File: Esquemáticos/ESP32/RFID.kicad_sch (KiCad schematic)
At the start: 1 part

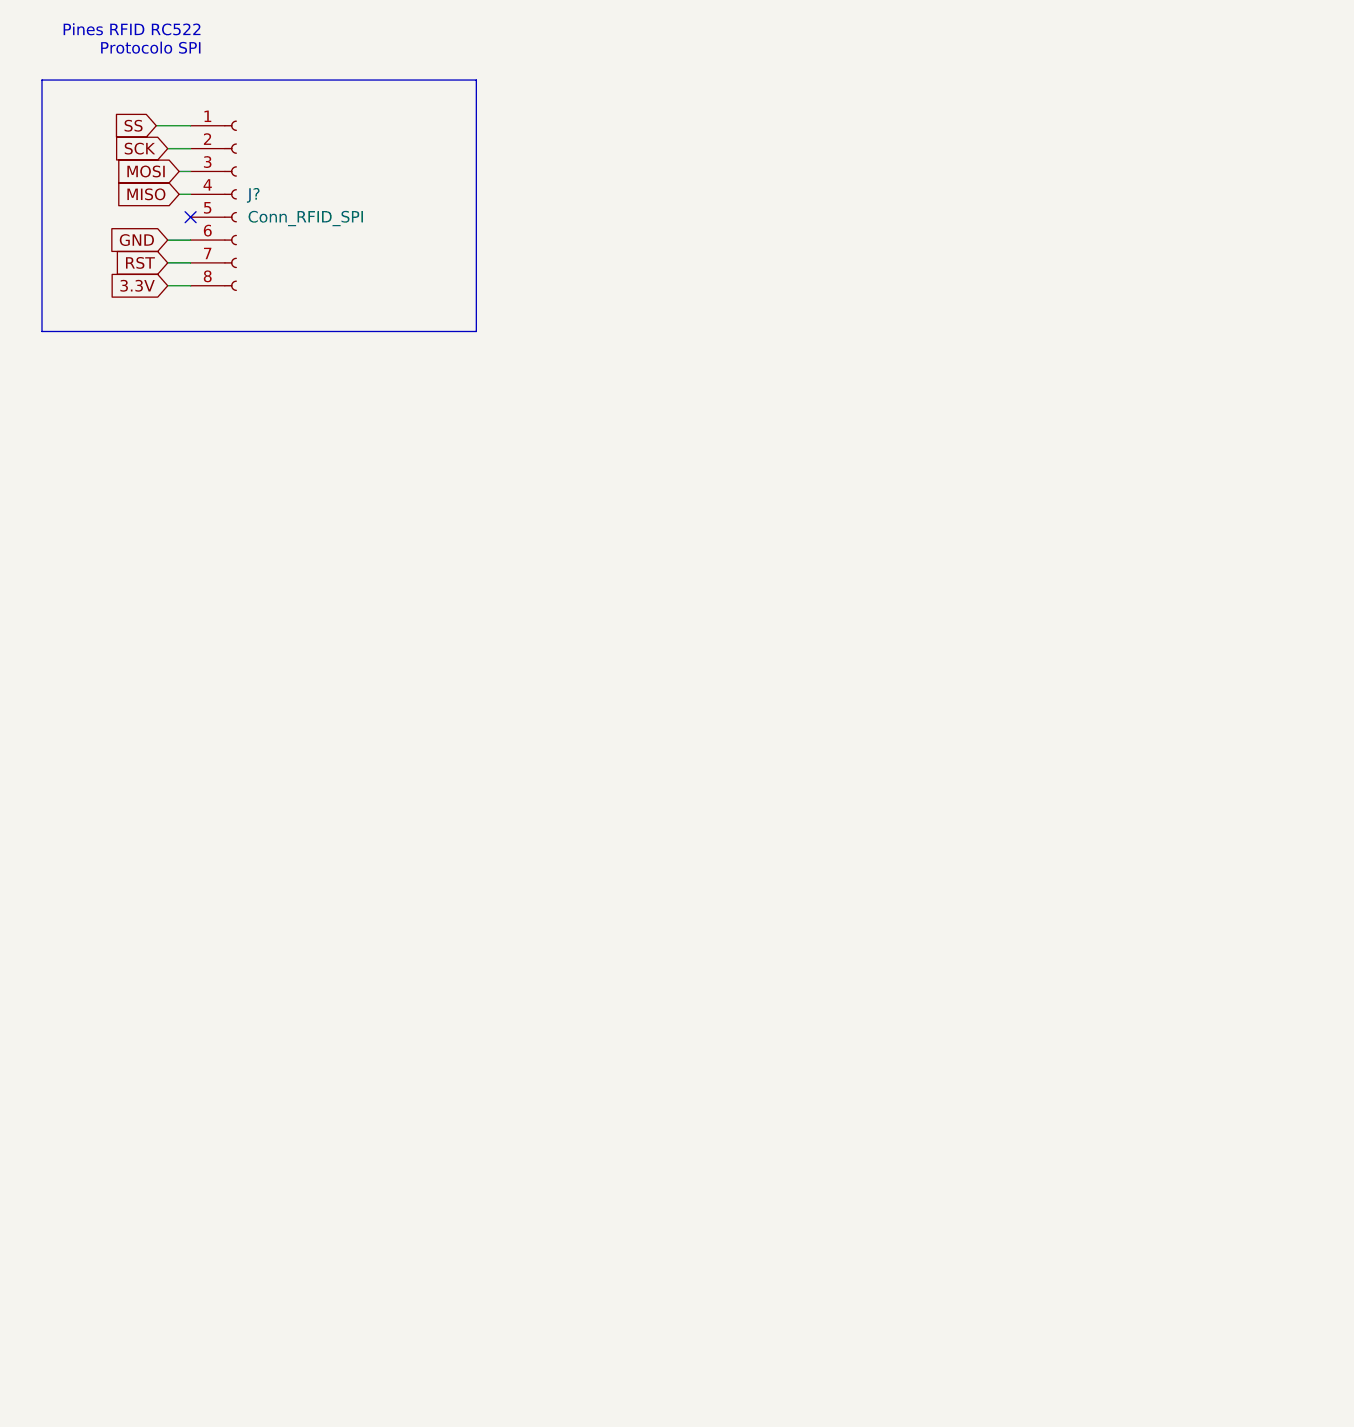
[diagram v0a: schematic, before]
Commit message: Cambios hechos al esquemático, faltan detalles
Revisar el discord para dejar todo al día con el feedback de hoy
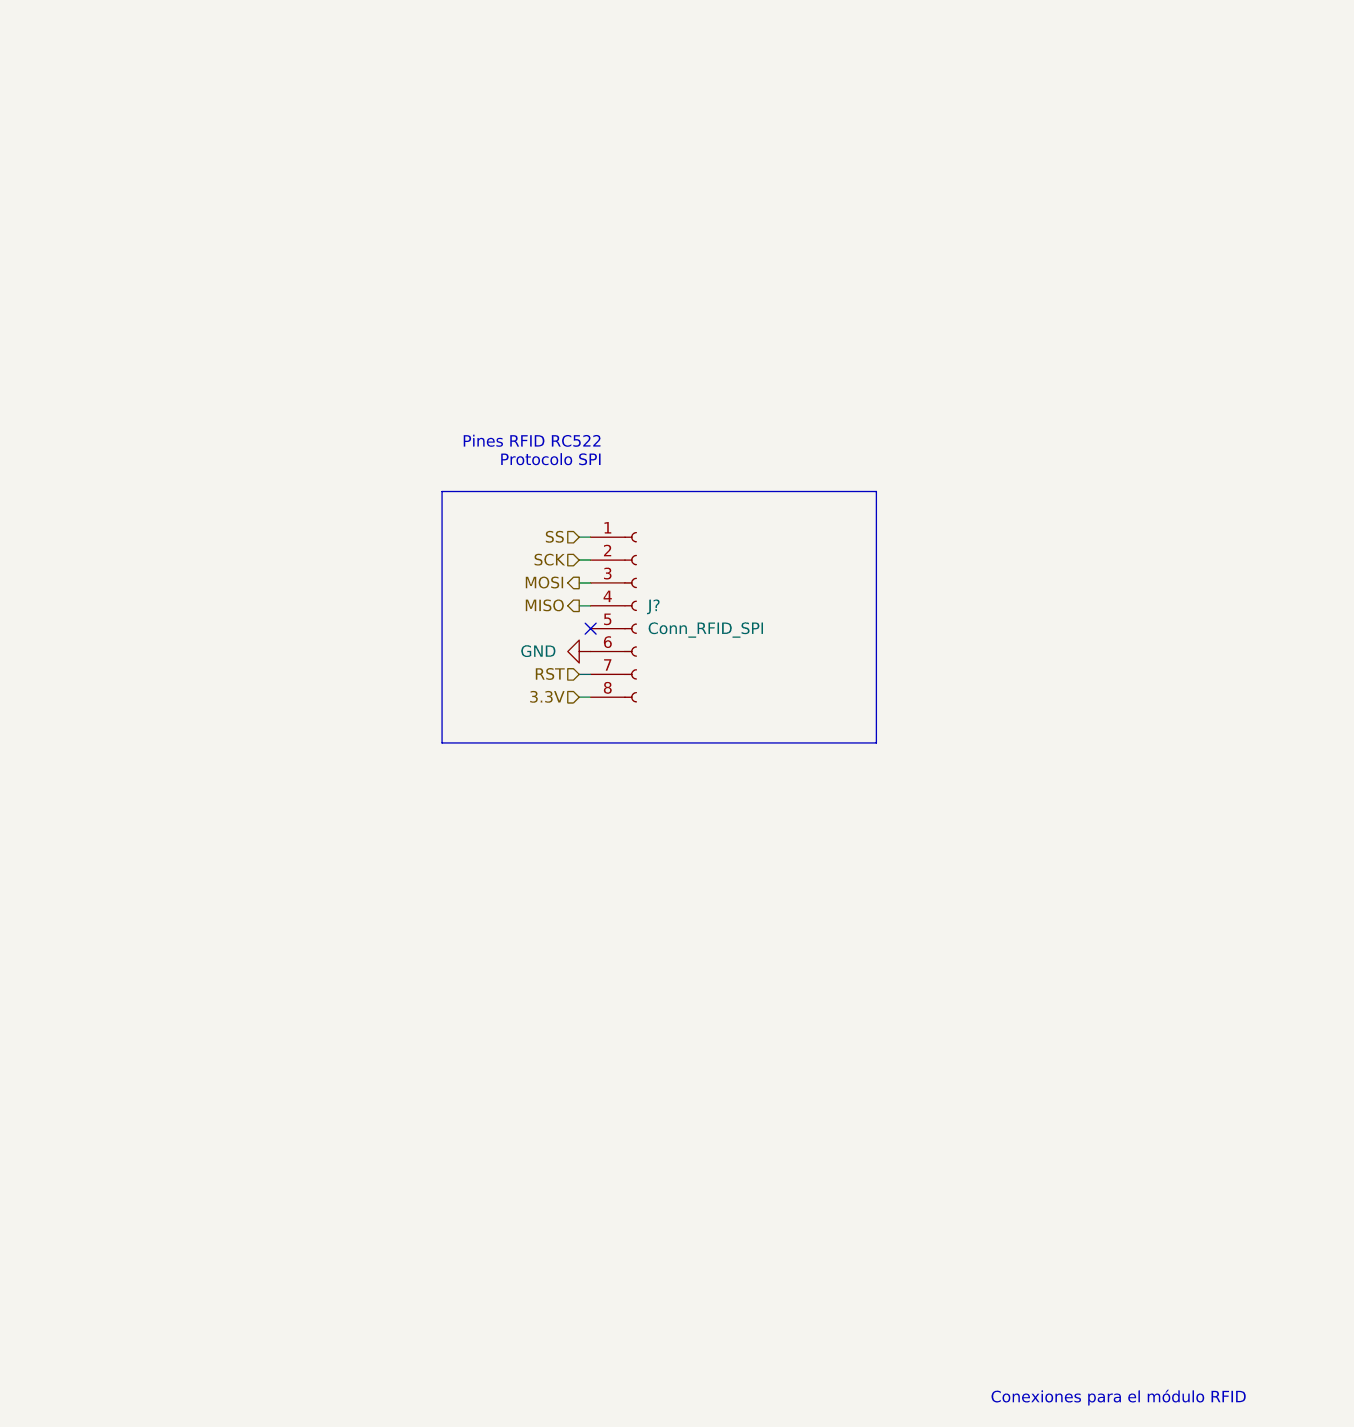
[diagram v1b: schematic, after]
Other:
- note added: "Conexiones para el módulo RFID"
- moved on the sheet: J?
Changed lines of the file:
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@@
 (kicad_sch (version 20211123) (generator eeschema)
   (paper "A4")
-  (no_connect (at 97.79 58.42))
-  (wire (pts (xy 95.25 50.8) (xy 97.79 50.8))
+  (no_connect (at 142.24 104.14))
+  (wire (pts (xy 140.97 96.52) (xy 142.24 96.52))
     (stroke (width 0) (type default) (color 0 0 0 0))
   )
-  (polyline (pts (xy 81.28 71.12) (xy 81.28 43.18))
+  (polyline (pts (xy 125.73 116.84) (xy 125.73 88.9))
     (stroke (width 0) (type default) (color 0 0 0 0))
   )
-  (wire (pts (xy 95.25 63.5) (xy 97.79 63.5))
+  (wire (pts (xy 140.97 109.22) (xy 142.24 109.22))
     (stroke (width 0) (type default) (color 0 0 0 0))
   )
-  (polyline (pts (xy 129.54 71.12) (xy 81.28 71.12))
+  (polyline (pts (xy 173.99 116.84) (xy 125.73 116.84))
     (stroke (width 0) (type default) (color 0 0 0 0))
   )
-  (wire (pts (xy 95.25 66.04) (xy 97.79 66.04))
+  (wire (pts (xy 140.97 111.76) (xy 142.24 111.76))
     (stroke (width 0) (type default) (color 0 0 0 0))
   )
-  (polyline (pts (xy 129.54 43.18) (xy 129.54 71.12))
+  (polyline (pts (xy 173.99 88.9) (xy 173.99 116.84))
     (stroke (width 0) (type default) (color 0 0 0 0))
   )
-  (wire (pts (xy 96.52 55.88) (xy 97.79 55.88))
+  (wire (pts (xy 140.97 101.6) (xy 142.24 101.6))
     (stroke (width 0) (type default) (color 0 0 0 0))
   )
-  (polyline (pts (xy 81.28 43.18) (xy 129.54 43.18))
+  (polyline (pts (xy 125.73 88.9) (xy 173.99 88.9))
     (stroke (width 0) (type default) (color 0 0 0 0))
   )
-  (wire (pts (xy 96.52 53.34) (xy 97.79 53.34))
+  (wire (pts (xy 140.97 99.06) (xy 142.24 99.06))
     (stroke (width 0) (type default) (color 0 0 0 0))
   )
-  (wire (pts (xy 95.25 60.96) (xy 97.79 60.96))
+  (wire (pts (xy 140.97 93.98) (xy 142.24 93.98))
     (stroke (width 0) (type default) (color 0 0 0 0))
   )
-  (wire (pts (xy 93.98 48.26) (xy 97.79 48.26))
-    (stroke (width 0) (type default) (color 0 0 0 0))
+  (text "Conexiones para el módulo RFID" (at 186.69 190.5 0)
+    (effects (font (size 1.27 1.27)) (justify left bottom))
   )
-  (text "Pines RFID RC522\nProtocolo SPI" (at 99.06 40.64 180)
+  (text "Pines RFID RC522\nProtocolo SPI" (at 143.51 86.36 180)
     (effects (font (size 1.27 1.27)) (justify right bottom))
   )
-  (global_label "MISO" (shape input) (at 96.52 55.88 180) (fields_autoplaced)
+  (hierarchical_label "MOSI" (shape output) (at 140.97 99.06 180)
     (effects (font (size 1.27 1.27)) (justify right))
-    (property "Referencias entre hojas" "${INTERSHEET_REFS}" (id 0) (at 89.5107 55.8006 0)
-      (effects (font (size 1.27 1.27)) (justify right) hide)
-    )
   )
-  (global_label "3.3V" (shape input) (at 95.25 66.04 180) (fields_autoplaced)
+  (hierarchical_label "MISO" (shape output) (at 140.97 101.6 180)
     (effects (font (size 1.27 1.27)) (justify right))
-    (property "Referencias entre hojas" "${INTERSHEET_REFS}" (id 0) (at 88.7245 65.9606 0)
-      (effects (font (size 1.27 1.27)) (justify right) hide)
-    )
   )
-  (global_label "SS" (shape input) (at 93.98 48.26 180) (fields_autoplaced)
+  (hierarchical_label "SS" (shape input) (at 140.97 93.98 180)
     (effects (font (size 1.27 1.27)) (justify right))
-    (property "Referencias entre hojas" "${INTERSHEET_REFS}" (id 0) (at 89.1479 48.1806 0)
-      (effects (font (size 1.27 1.27)) (justify right) hide)
-    )
   )
-  (global_label "MOSI" (shape input) (at 96.52 53.34 180) (fields_autoplaced)
+  (hierarchical_label "SCK" (shape input) (at 140.97 96.52 180)
     (effects (font (size 1.27 1.27)) (justify right))
-    (property "Referencias entre hojas" "${INTERSHEET_REFS}" (id 0) (at 89.5107 53.2606 0)
-      (effects (font (size 1.27 1.27)) (justify right) hide)
-    )
   )
-  (global_label "RST" (shape input) (at 95.25 63.5 180) (fields_autoplaced)
+  (hierarchical_label "3.3V" (shape input) (at 140.97 111.76 180)
     (effects (font (size 1.27 1.27)) (justify right))
-    (property "Referencias entre hojas" "${INTERSHEET_REFS}" (id 0) (at 89.3898 63.4206 0)
-      (effects (font (size 1.27 1.27)) (justify right) hide)
-    )
   )
-  (global_label "GND" (shape input) (at 95.25 60.96 180) (fields_autoplaced)
+  (hierarchical_label "RST" (shape input) (at 140.97 109.22 180)
     (effects (font (size 1.27 1.27)) (justify right))
-    (property "Referencias entre hojas" "${INTERSHEET_REFS}" (id 0) (at 88.9664 60.8806 0)
-      (effects (font (size 1.27 1.27)) (justify right) hide)
-    )
   )
-  (global_label "SCK" (shape input) (at 95.25 50.8 180) (fields_autoplaced)
-    (effects (font (size 1.27 1.27)) (justify right))
-    (property "Referencias entre hojas" "${INTERSHEET_REFS}" (id 0) (at 89.0874 50.7206 0)
-      (effects (font (size 1.27 1.27)) (justify right) hide)
-    )
-  )
-  (symbol (lib_id "Connector:Conn_01x08_Female") (at 102.87 55.88 0) (unit 1)
+  (symbol (lib_id "Connector:Conn_01x08_Female") (at 147.32 101.6 0) (unit 1)
     (in_bom yes) (on_board yes) (fields_autoplaced)
-    (property "Reference" "J?" (id 0) (at 104.14 55.8799 0)
+    (property "Reference" "J?" (id 0) (at 148.59 101.5999 0)
       (effects (font (size 1.27 1.27)) (justify left))
     )
-    (property "Value" "Conn_RFID_SPI" (id 1) (at 104.14 58.4199 0)
+    (property "Value" "Conn_RFID_SPI" (id 1) (at 148.59 104.1399 0)
       (effects (font (size 1.27 1.27)) (justify left))
     )
-    (property "Footprint" "" (id 2) (at 102.87 55.88 0)
+    (property "Footprint" "" (id 2) (at 147.32 101.6 0)
       (effects (font (size 1.27 1.27)) hide)
     )
-    (property "Datasheet" "~" (id 3) (at 102.87 55.88 0)
+    (property "Datasheet" "~" (id 3) (at 147.32 101.6 0)
       (effects (font (size 1.27 1.27)) hide)
     )
@@
     (pin "8")
   )
+  (symbol (lib_id "power:GND") (at 142.24 106.68 270) (unit 1)
+    (in_bom yes) (on_board yes) (fields_autoplaced)
+    (property "Reference" "#PWR?" (id 0) (at 135.89 106.68 0)
+      (effects (font (size 1.27 1.27)) hide)
+    )
+    (property "Value" "GND" (id 1) (at 138.43 106.6799 90)
+      (effects (font (size 1.27 1.27)) (justify right))
+    )
+    (property "Footprint" "" (id 2) (at 142.24 106.68 0)
+      (effects (font (size 1.27 1.27)) hide)
+    )
+    (property "Datasheet" "" (id 3) (at 142.24 106.68 0)
+      (effects (font (size 1.27 1.27)) hide)
+    )
+    (pin "1")
+  )
 )

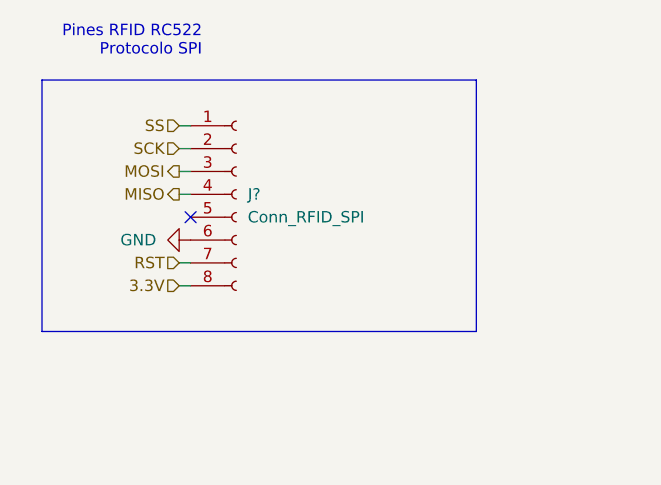
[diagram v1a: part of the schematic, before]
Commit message: actualización raul
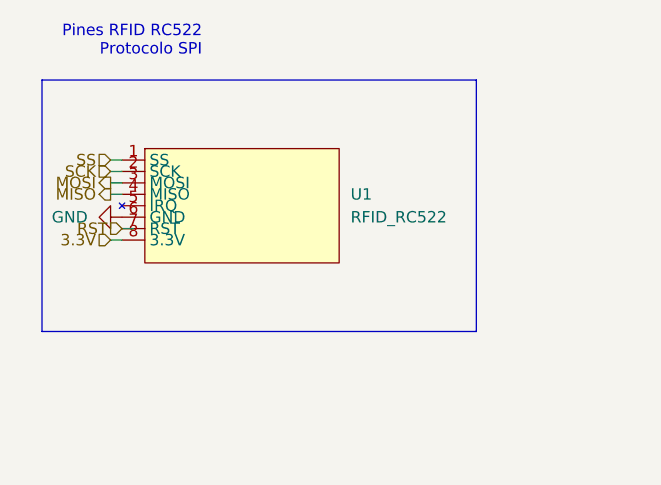
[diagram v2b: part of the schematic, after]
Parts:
- removed J?: Conn_RFID_SPI, symbol Connector:Conn_01x08_Female
- added U1: RFID_RC522, symbol libreria_raul:RFID_RC522
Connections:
- net 3.3V: now also U1.8 (3.3V)
- net GND: now also U1.6 (GND)
- net MISO: now also U1.4 (MISO)
- net MOSI: now also U1.3 (MOSI)
- net RST: now also U1.7 (RST)
- net SCK: now also U1.2 (SCK)
- net SS: now also U1.1 (SS)
- no-connect marks 1 -> 0
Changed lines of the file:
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@@
 (kicad_sch (version 20211123) (generator eeschema)
   (paper "A4")
-  (no_connect (at 142.24 104.14))
-  (wire (pts (xy 140.97 96.52) (xy 142.24 96.52))
+  (wire (pts (xy 133.35 99.06) (xy 134.62 99.06))
     (stroke (width 0) (type default) (color 0 0 0 0))
   )
@@
     (stroke (width 0) (type default) (color 0 0 0 0))
   )
-  (wire (pts (xy 140.97 109.22) (xy 142.24 109.22))
+  (wire (pts (xy 134.62 105.41) (xy 135.89 105.41))
     (stroke (width 0) (type default) (color 0 0 0 0))
   )
@@
     (stroke (width 0) (type default) (color 0 0 0 0))
   )
-  (wire (pts (xy 140.97 111.76) (xy 142.24 111.76))
+  (wire (pts (xy 133.35 106.68) (xy 134.62 106.68))
     (stroke (width 0) (type default) (color 0 0 0 0))
   )
@@
     (stroke (width 0) (type default) (color 0 0 0 0))
   )
-  (wire (pts (xy 140.97 101.6) (xy 142.24 101.6))
+  (wire (pts (xy 133.35 101.6) (xy 134.62 101.6))
     (stroke (width 0) (type default) (color 0 0 0 0))
   )
@@
     (stroke (width 0) (type default) (color 0 0 0 0))
   )
-  (wire (pts (xy 140.97 99.06) (xy 142.24 99.06))
+  (wire (pts (xy 133.35 100.33) (xy 134.62 100.33))
     (stroke (width 0) (type default) (color 0 0 0 0))
   )
-  (wire (pts (xy 140.97 93.98) (xy 142.24 93.98))
+  (wire (pts (xy 133.35 97.79) (xy 134.62 97.79))
     (stroke (width 0) (type default) (color 0 0 0 0))
   )
@@
     (effects (font (size 1.27 1.27)) (justify right bottom))
   )
-  (hierarchical_label "MOSI" (shape output) (at 140.97 99.06 180)
+  (hierarchical_label "MOSI" (shape output) (at 133.35 100.33 180)
     (effects (font (size 1.27 1.27)) (justify right))
   )
-  (hierarchical_label "MISO" (shape output) (at 140.97 101.6 180)
+  (hierarchical_label "MISO" (shape output) (at 133.35 101.6 180)
     (effects (font (size 1.27 1.27)) (justify right))
   )
-  (hierarchical_label "SS" (shape input) (at 140.97 93.98 180)
+  (hierarchical_label "SS" (shape input) (at 133.35 97.79 180)
     (effects (font (size 1.27 1.27)) (justify right))
   )
-  (hierarchical_label "SCK" (shape input) (at 140.97 96.52 180)
+  (hierarchical_label "SCK" (shape input) (at 133.35 99.06 180)
     (effects (font (size 1.27 1.27)) (justify right))
   )
-  (hierarchical_label "3.3V" (shape input) (at 140.97 111.76 180)
+  (hierarchical_label "3.3V" (shape input) (at 133.35 106.68 180)
     (effects (font (size 1.27 1.27)) (justify right))
   )
-  (hierarchical_label "RST" (shape input) (at 140.97 109.22 180)
+  (hierarchical_label "RST" (shape input) (at 134.62 105.41 180)
     (effects (font (size 1.27 1.27)) (justify right))
   )
-  (symbol (lib_id "Connector:Conn_01x08_Female") (at 147.32 101.6 0) (unit 1)
+  (symbol (lib_id "libreria_raul:RFID_RC522") (at 146.05 93.98 0) (unit 1)
     (in_bom yes) (on_board yes) (fields_autoplaced)
-    (property "Reference" "J?" (id 0) (at 148.59 101.5999 0)
+    (property "Reference" "U1" (id 0) (at 160.02 101.5999 0)
       (effects (font (size 1.27 1.27)) (justify left))
     )
-    (property "Value" "Conn_RFID_SPI" (id 1) (at 148.59 104.1399 0)
+    (property "Value" "RFID_RC522" (id 1) (at 160.02 104.1399 0)
       (effects (font (size 1.27 1.27)) (justify left))
     )
-    (property "Footprint" "" (id 2) (at 147.32 101.6 0)
+    (property "Footprint" "" (id 2) (at 146.05 93.98 0)
       (effects (font (size 1.27 1.27)) hide)
     )
-    (property "Datasheet" "~" (id 3) (at 147.32 101.6 0)
+    (property "Datasheet" "" (id 3) (at 146.05 93.98 0)
       (effects (font (size 1.27 1.27)) hide)
     )
@@
     (pin "8")
   )
-  (symbol (lib_id "power:GND") (at 142.24 106.68 270) (unit 1)
+  (symbol (lib_id "power:GND") (at 134.62 104.14 270) (unit 1)
     (in_bom yes) (on_board yes) (fields_autoplaced)
-    (property "Reference" "#PWR?" (id 0) (at 135.89 106.68 0)
+    (property "Reference" "#PWR?" (id 0) (at 128.27 104.14 0)
       (effects (font (size 1.27 1.27)) hide)
     )
-    (property "Value" "GND" (id 1) (at 138.43 106.6799 90)
+    (property "Value" "GND" (id 1) (at 130.81 104.1399 90)
       (effects (font (size 1.27 1.27)) (justify right))
     )
-    (property "Footprint" "" (id 2) (at 142.24 106.68 0)
+    (property "Footprint" "" (id 2) (at 134.62 104.14 0)
       (effects (font (size 1.27 1.27)) hide)
     )
-    (property "Datasheet" "" (id 3) (at 142.24 106.68 0)
+    (property "Datasheet" "" (id 3) (at 134.62 104.14 0)
       (effects (font (size 1.27 1.27)) hide)
     )
